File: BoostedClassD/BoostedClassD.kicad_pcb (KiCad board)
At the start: 4 copper layers, 66.5 x 53.3 mm, 71 parts, among them IC1 BQ25185, IC2 ESP32-WROOM-32UE-N8R2, IC3 RESET, IC4 BOOT, IC5 INA236, J1 SYSTEM CONNECTOR 1, J2 SYSTEM CONNECTOR 2, J3 SPK OUT, J4 PROG, Q1 DMG3415U, U1 TPS631000, U2 TAS2320, U3 TAS2120, U4 TPS7A2018, U5 ATtiny412

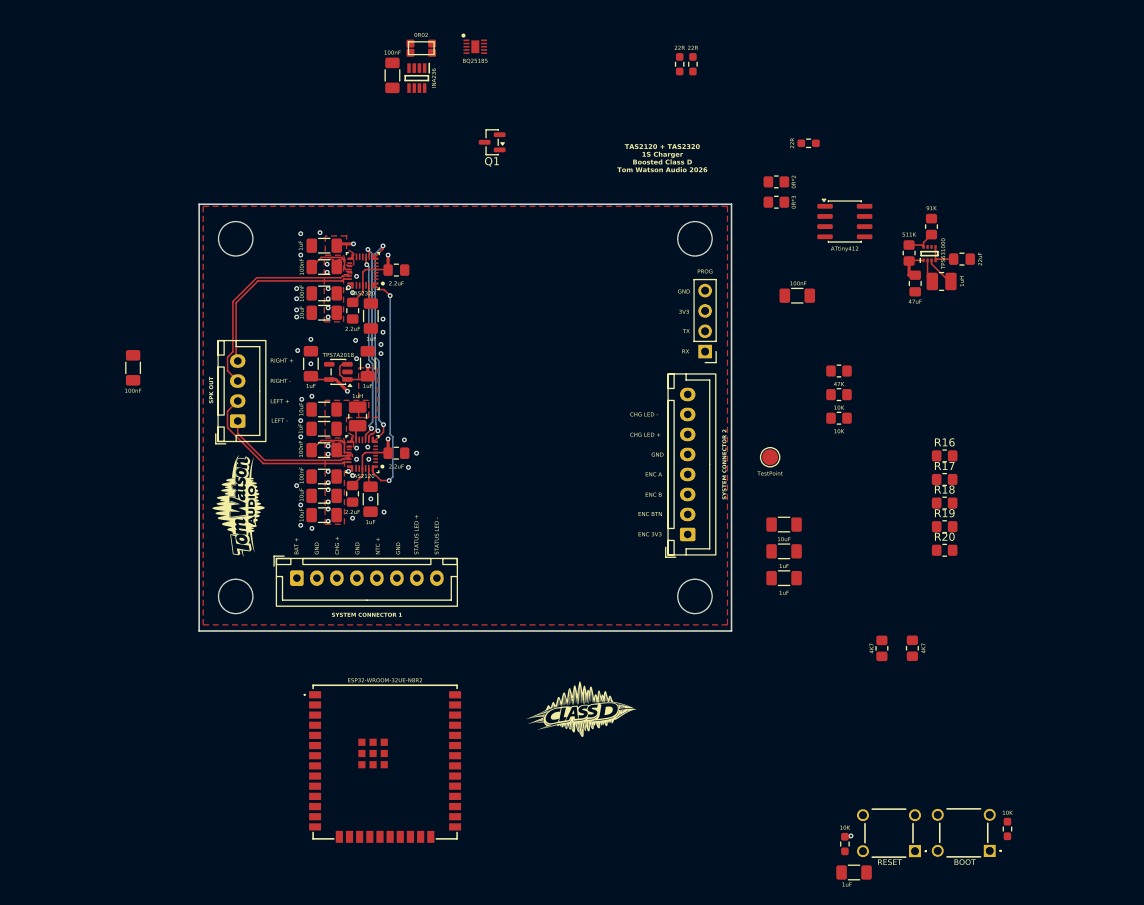
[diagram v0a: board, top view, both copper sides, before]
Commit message: more
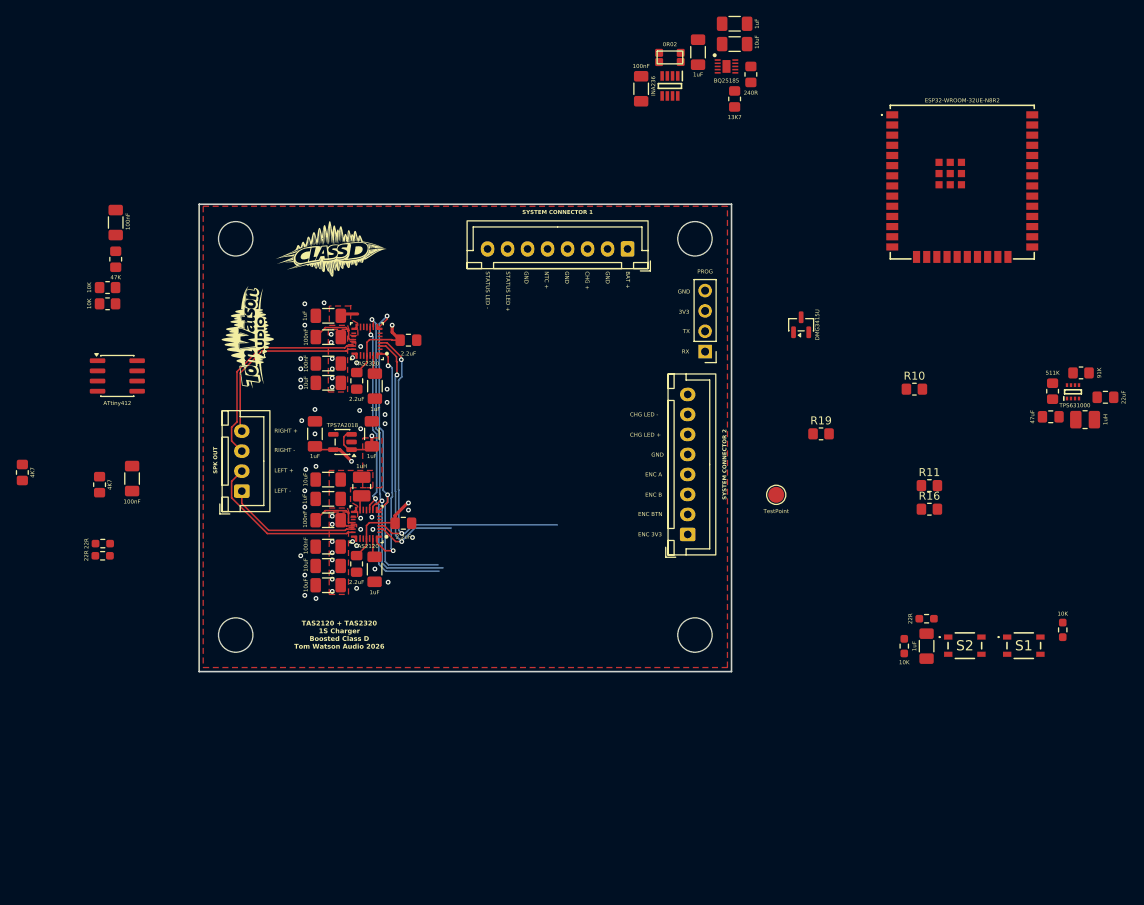
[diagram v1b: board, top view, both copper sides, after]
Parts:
- removed IC3: RESET, Custom:TS026650BK100SCRD
- removed IC4: BOOT, Custom:TS026650BK100SCRD
- removed R20: 2K2, Resistor_SMD:R_0805_2012Metric_Pad1.20x1.40mm_HandSolder
- added S1: BOOT, Custom:PTS810SJM250SMTRLFS, F.Cu at (219.4, 126.6)
- added S2: EN, Custom:PTS810SJM250SMTRLFS, F.Cu at (212.0, 126.6)
- moved R8 113.4 mm to (94.2, 104.9), turned to -90 degrees
- moved IC2 102.3 mm to (211.7, 68.9)
- moved R12 99.9 mm to (103.9, 106.4), turned to -90 degrees
- moved R3 95.0 mm to (104.3, 113.8), turned to 0 degrees
- moved R4 94.8 mm to (104.3, 115.3), turned to 0 degrees
- moved U5 93.0 mm to (106.1, 92.8)
- moved R15 92.5 mm to (104.9, 83.8)
- moved R14 92.4 mm to (104.9, 81.8)
- moved R13 91.5 mm to (105.9, 78.2), turned to -90 degrees
- moved C8 85.7 mm to (105.9, 73.7), turned to 90 degrees
- moved C27 66.6 mm to (178.7, 52.4), turned to 90 degrees
- moved C26 66.2 mm to (183.3, 48.8), turned to 180 degrees
- moved G*** 65.5 mm to (132.8, 77.5)
- moved R5 61.2 mm to (207.3, 123.2)
- moved C25 60.4 mm to (183.3, 51.4)
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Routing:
- net /Amplifiers/SCL: track 0.00 -> 48.8 mm, vias 0 -> 2
- net /Amplifiers/SDA: track 0.00 -> 36.5 mm, vias 0 -> 2
- net /Amplifiers/DATA: track 23.9 -> 40.1 mm
- net /Amplifiers/BCK: track 26.0 -> 41.7 mm
- net /Amplifiers/LRCK: track 28.2 -> 43.4 mm
- net /ENC 3V3: track 5.21 -> 0.00 mm, vias 1 -> 0
- net Net-(U1-FB): track 3.85 -> 0.00 mm
- net Net-(U1-LX1): track 3.78 -> 0.00 mm
- net /Amplifiers/SYS: track 29.7 -> 26.3 mm, vias 2 -> 1
- net /Amplifiers/VDD1V8: track 53.0 -> 55.9 mm
- net Net-(U1-LX2): track 2.89 -> 0.00 mm
- net /ENC A: track 0.61 -> 0.00 mm
- net GND: vias 39 -> 38
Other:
- board size 66.5 x 53.3 mm -> 66.5 x 58.4 mm
